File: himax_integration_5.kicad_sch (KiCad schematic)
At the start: 29 parts, among them J1 VBat, J2 GND Pad, J3 SWDCLK Pad, J4 SWDIO Pad, J5 RST Pad, J6 Antenna Pad, Q2 Q_NPN, U1 ICM-42688-P, U2 MAG_Switch, U3 ES2832AA2

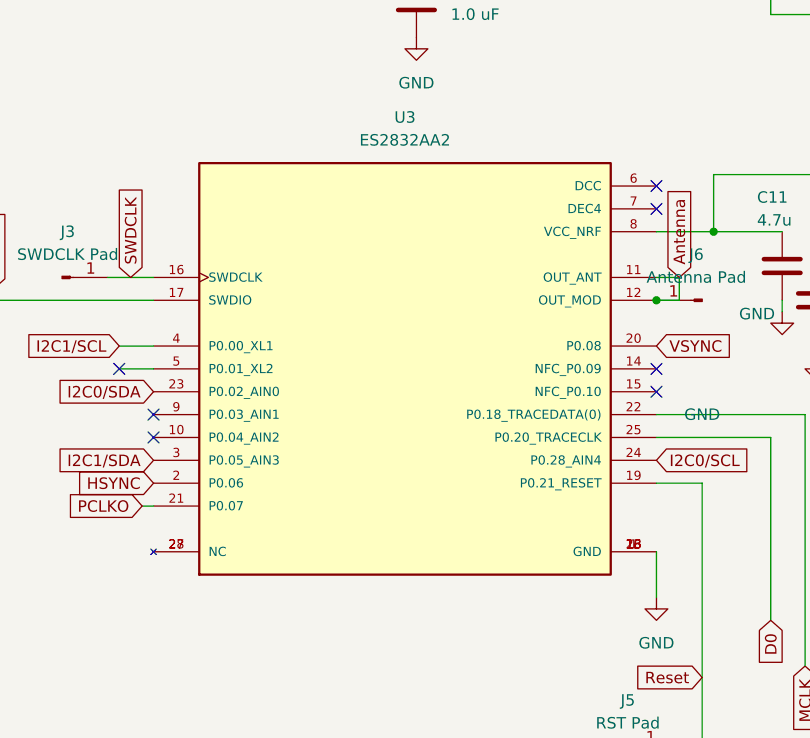
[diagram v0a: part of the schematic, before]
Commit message: restructured with local libs
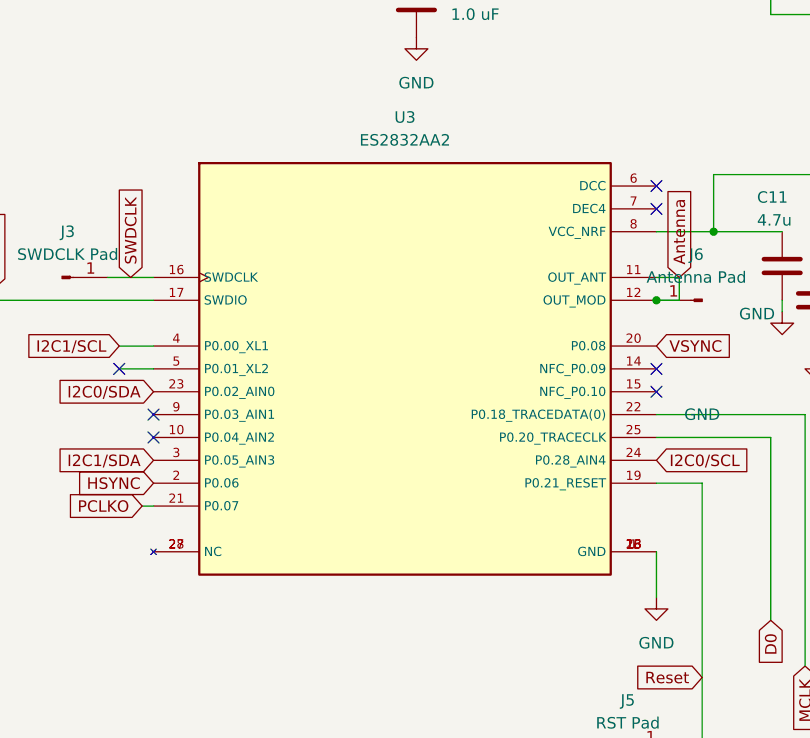
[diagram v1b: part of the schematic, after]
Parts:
- HM01B1: footprint camera_flexa:camerah -> HM01B0:camerah
- J1, J2, J3, J4, J5, J6: footprint Connector_Pin:ExternalPad_FP -> himax_custom:ExternalPad_FP; symbol Connector:ExternalPad1 -> himax_custom:ExternalPad1
- Q2: footprint Package_TO_SOT_SMD:SOT-883_1 -> himax_custom:SOT-883_1
- U2: footprint kicad_fp_sch_vreg:RR122 -> RR122:RR122
- U3: footprint ES2832AA2 (1):XCVR_ES2832AA2 -> ES2832AA2:XCVR_ES2832AA2_NO_ANTENNA; symbol ES2832AA2:ES2832AA2 -> ES2832AA2:ES2832AA2_NO_ANTENNA
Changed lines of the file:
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@@
 	)
 	(symbol
-		(lib_id "Connector:ExternalPad1")
+		(lib_id "himax_custom:ExternalPad1")
 		(at 165.1 99.06 180)
 		(unit 1)
@@
 			)
 		)
-		(property "Footprint" "Connector_Pin:ExternalPad_FP"
+		(property "Footprint" "himax_custom:ExternalPad_FP"
 			(at 165.1 99.06 0)
 			(hide yes)
@@
 	)
 	(symbol
-		(lib_id "Connector:ExternalPad1")
+		(lib_id "himax_custom:ExternalPad1")
 		(at 156.21 148.59 0)
 		(unit 1)
@@
 			)
 		)
-		(property "Footprint" "Connector_Pin:ExternalPad_FP"
+		(property "Footprint" "himax_custom:ExternalPad_FP"
 			(at 156.21 148.59 0)
 			(hide yes)
@@
 	)
 	(symbol
-		(lib_id "Connector:ExternalPad1")
+		(lib_id "himax_custom:ExternalPad1")
 		(at 93.98 96.52 0)
 		(unit 1)
@@
 			)
 		)
-		(property "Footprint" "Connector_Pin:ExternalPad_FP"
+		(property "Footprint" "himax_custom:ExternalPad_FP"
 			(at 93.98 96.52 0)
 			(hide yes)
@@
 			)
 		)
-		(property "Footprint" "kicad_fp_sch_vreg:RR122"
+		(property "Footprint" "RR122:RR122"
 			(at 201.93 55.88 0)
 			(hide yes)
@@
 	)
 	(symbol
-		(lib_id "Connector:ExternalPad1")
+		(lib_id "himax_custom:ExternalPad1")
 		(at 76.2 99.06 0)
 		(unit 1)
@@
 			)
 		)
-		(property "Footprint" "Connector_Pin:ExternalPad_FP"
+		(property "Footprint" "himax_custom:ExternalPad_FP"
 			(at 76.2 99.06 0)
 			(hide yes)
@@
 	)
 	(symbol
-		(lib_id "Connector:ExternalPad1")
+		(lib_id "himax_custom:ExternalPad1")
 		(at 201.93 40.64 270)
 		(unit 1)
@@
 			)
 		)
-		(property "Footprint" "Connector_Pin:ExternalPad_FP"
+		(property "Footprint" "himax_custom:ExternalPad_FP"
 			(at 201.93 40.64 0)
 			(hide yes)
@@
 	)
 	(symbol
-		(lib_id "Connector:ExternalPad1")
+		(lib_id "himax_custom:ExternalPad1")
 		(at 236.22 20.32 270)
 		(unit 1)
@@
 			)
 		)
-		(property "Footprint" "Connector_Pin:ExternalPad_FP"
+		(property "Footprint" "himax_custom:ExternalPad_FP"
 			(at 236.22 20.32 0)
 			(hide yes)
@@
 			)
 		)
-		(property "Footprint" "Package_TO_SOT_SMD:SOT-883_1"
+		(property "Footprint" "himax_custom:SOT-883_1"
 			(at 43.18 170.18 0)
 			(hide yes)
@@
 			)
 		)
-		(property "Footprint" "camera_flexa:camerah"
+		(property "Footprint" "HM01B0:camerah"
 			(at 43.18 123.19 0)
 			(hide yes)
@@
 	)
 	(symbol
-		(lib_id "ES2832AA2:ES2832AA2")
+		(lib_id "ES2832AA2:ES2832AA2_NO_ANTENNA")
 		(at 132.08 106.68 0)
 		(unit 1)
@@
 			)
 		)
-		(property "Footprint" "ES2832AA2 (1):XCVR_ES2832AA2"
-			(at 132.08 106.68 0)
+		(property "Footprint" "ES2832AA2:XCVR_ES2832AA2_NO_ANTENNA"
+			(at 128.27 77.47 0)
 			(hide yes)
 			(show_name no)
@@
 					(size 1.27 1.27)
 				)
-				(justify bottom)
 			)
 		)
 		(property "Datasheet" ""
-			(at 132.08 106.68 0)
+			(at 128.27 77.47 0)
 			(hide yes)
 			(show_name no)
@@
 		)
 		(property "Description" ""
-			(at 132.08 106.68 0)
+			(at 128.27 77.47 0)
 			(hide yes)
 			(show_name no)
